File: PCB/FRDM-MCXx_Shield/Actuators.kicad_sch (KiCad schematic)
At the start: 2 parts, among them IC2 STPIC6C595MTR

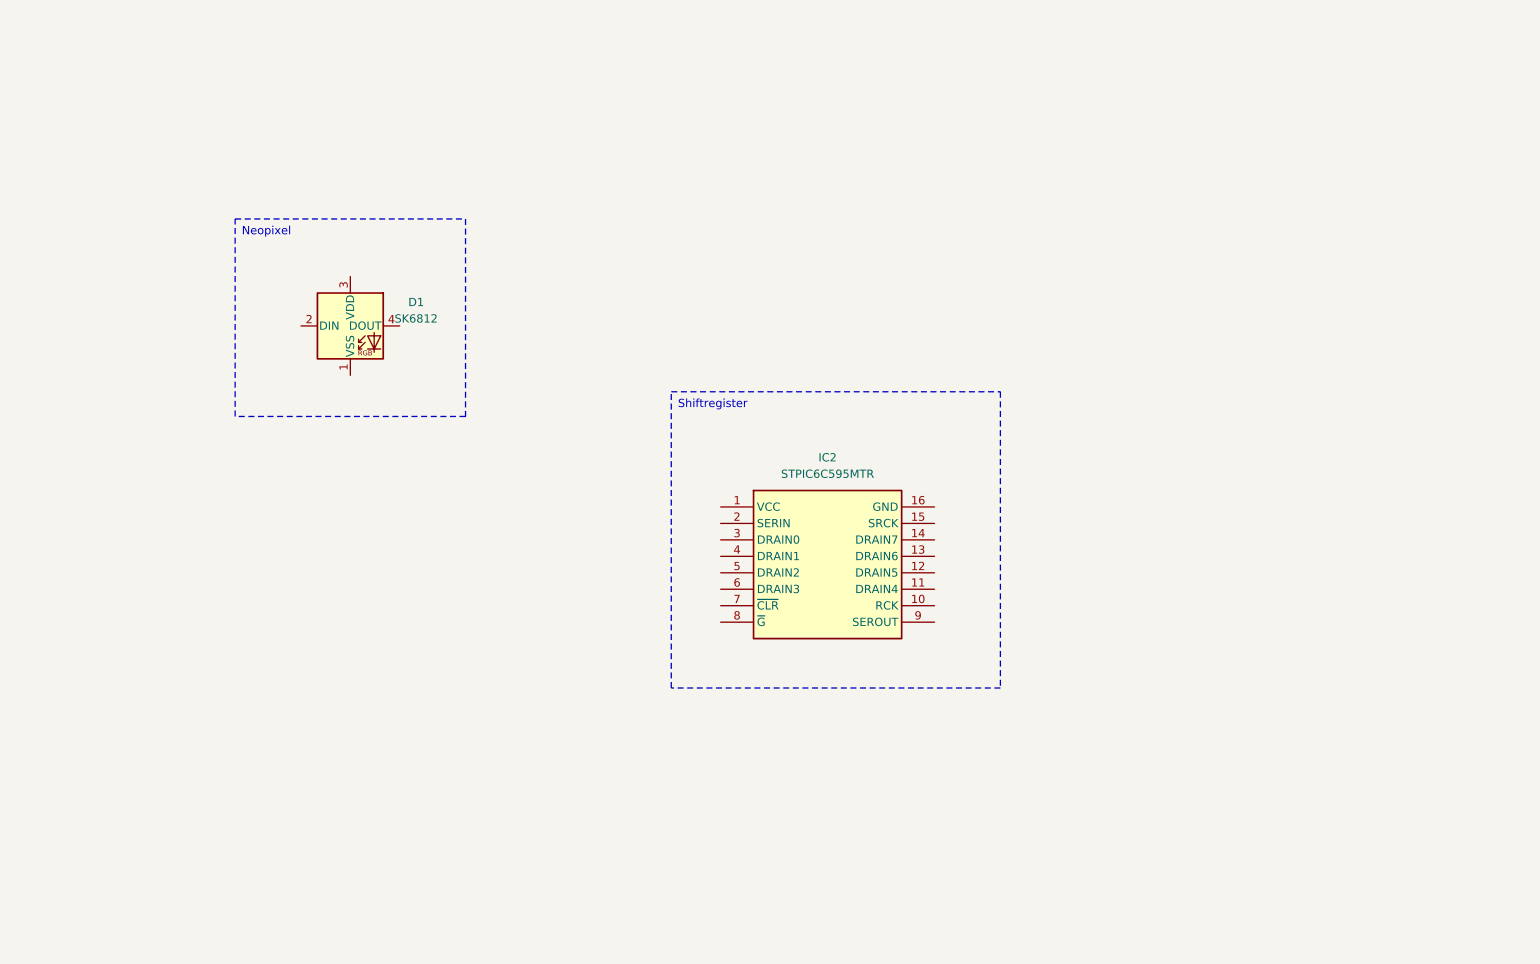
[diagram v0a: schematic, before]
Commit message: Updated schematic
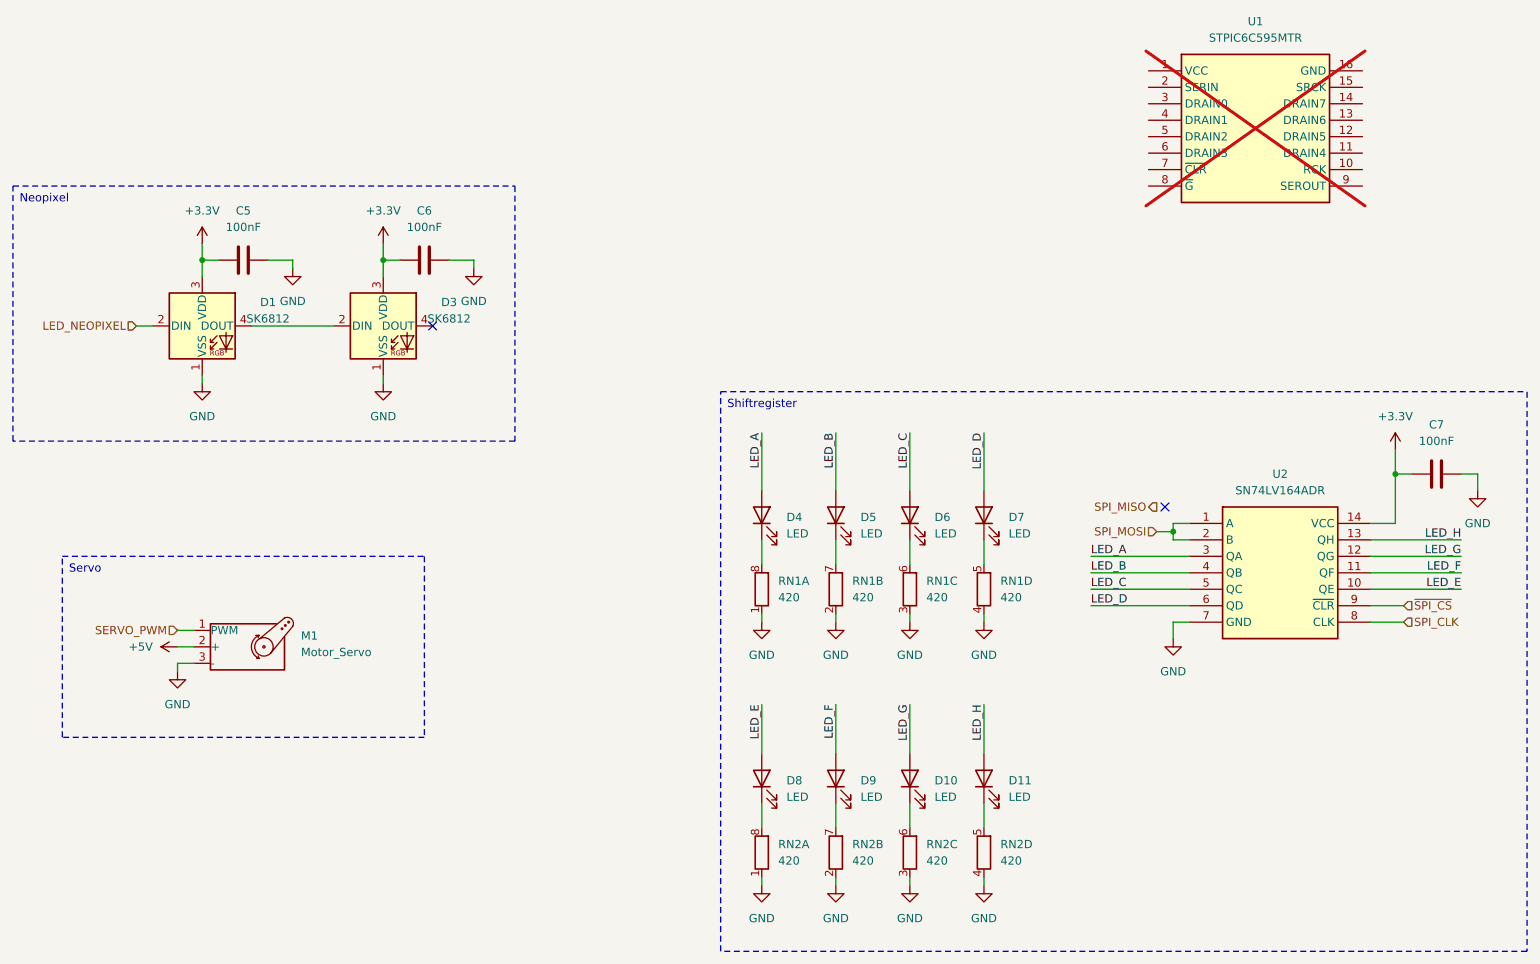
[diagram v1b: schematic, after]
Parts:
- removed IC2: STPIC6C595MTR, SOIC127P600X175-16N, symbol SamacSys_Parts:STPIC6C595MTR
- added C5, C6, C7: 100nF, Capacitor_SMD:C_0603_1608Metric_Pad1.08x0.95mm_HandSolder, symbol Device:C
- added D10, D11, D4, D5, D6, D7, D8, D9: LED, LED_SMD:LED_0603_1608Metric_Pad1.05x0.95mm_HandSolder, symbol Device:LED
- added D3: SK6812, LED_SMD:LED_SK6812_PLCC4_5.0x5.0mm_P3.2mm, symbol LED:SK6812
- added M1: Motor_Servo, Connector_PinHeader_2.54mm:PinHeader_1x03_P2.54mm_Vertical, symbol Motor:Motor_Servo
- added RN1, RN2: 420, Resistor_SMD:R_Array_Convex_4x0603, symbol Device:R_Pack04_Split
- added U1: STPIC6C595MTR, SOIC127P600X175-16N, symbol SamacSys_Parts:STPIC6C595MTR
- added U2: SN74LV164ADR, SOIC127P600X175-14N, symbol SamacSys_Parts:SN74LV164ADR
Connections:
- net GND: now reaches D1.1 (VSS)
- net GND: now also C5.2, C6.2, C7.2, D3.1 (VSS), M1.3 (-), RN1.1 (R1.1), RN1.2 (R2.1), RN1.3 (R3.1), RN1.4 (R4.1), RN2.1 (R1.1), RN2.2 (R2.1), RN2.3 (R3.1), RN2.4 (R4.1), U2.7 (GND)
- net LED_NEOPIXEL: now reaches D1.2 (DIN)
- net +3.3V: now reaches D1.3 (VDD)
- net +3.3V: now also C5.1, C6.1, C7.1, D3.3 (VDD), U2.14 (VCC)
- net at D1.4 (DOUT): now also D3.2 (DIN)
- new net: D5.1 (K), RN1.7 (R2.2)
- new net: D7.1 (K), RN1.5 (R4.2)
- new net: D8.1 (K), RN2.8 (R1.2)
- new net: D10.1 (K), RN2.6 (R3.2)
- new net: D4.1 (K), RN1.8 (R1.2)
- new net: D6.1 (K), RN1.6 (R3.2)
- new net: D11.1 (K), RN2.5 (R4.2)
- new net: D9.1 (K), RN2.7 (R2.2)
- new net +5V: M1.2 (+)
- new net LED_A: D4.2 (A), U2.3 (QA)
- new net LED_B: D5.2 (A), U2.4 (QB)
- new net LED_C: D6.2 (A), U2.5 (QC)
- new net LED_D: D7.2 (A), U2.6 (QD)
- new net LED_E: D8.2 (A), U2.10 (QE)
- new net LED_F: D9.2 (A), U2.11 (QF)
- new net LED_G: D10.2 (A), U2.12 (QG)
- new net LED_H: D11.2 (A), U2.13 (QH)
- new net SERVO_PWM: M1.1 (PWM)
- new net SPI_CLK: U2.8 (CLK)
- new net SPI_MOSI: U2.1 (A), U2.2 (B)
- new net ~{SPI_CS}: U2.9 (~{CLR})
- no-connect marks 0 -> 2
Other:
- company: (none) -> HAN
- title: (none) -> Actuators
- moved on the sheet: D1
